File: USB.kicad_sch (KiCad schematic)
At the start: 31 parts, among them J5 USB_C_Receptacle, J6 USB_C_Receptacle, SW1 SW_DIP_x04, U10 TPS2552, U11 TPD4EUSB30, U12 TPD4EUSB30, U13 TPD4EUSB30, U14 TPD4EUSB30, U15 TS3USB221, U16 HD3SS3220, U17 TS3USB221

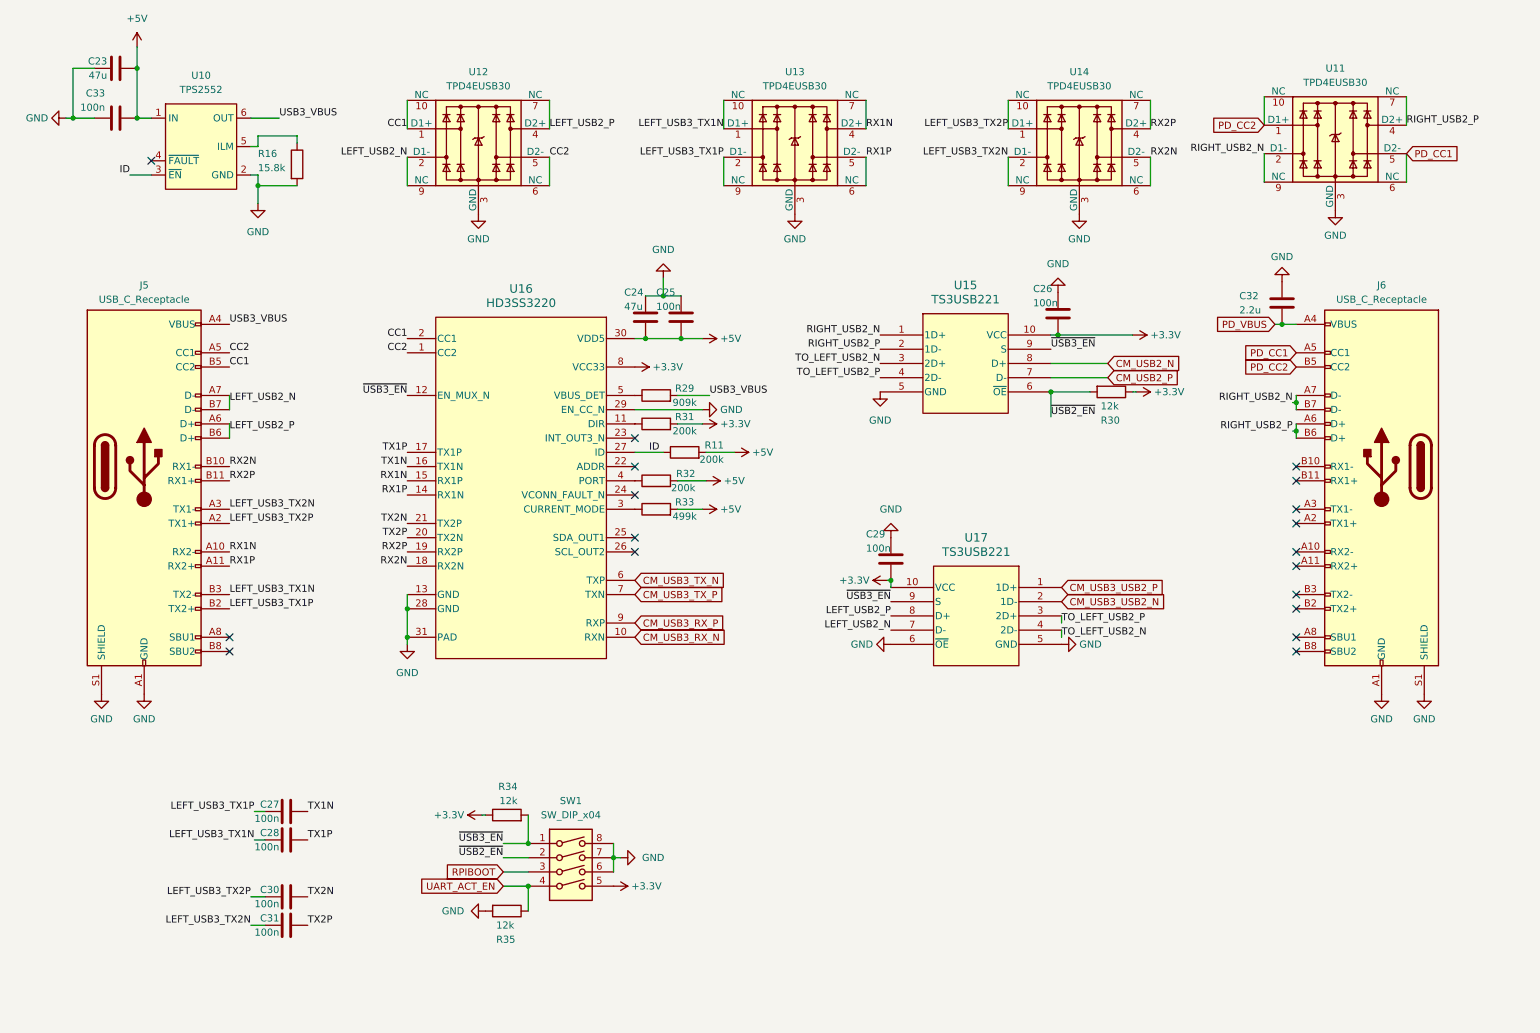
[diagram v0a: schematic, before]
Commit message: PiCard v3.0
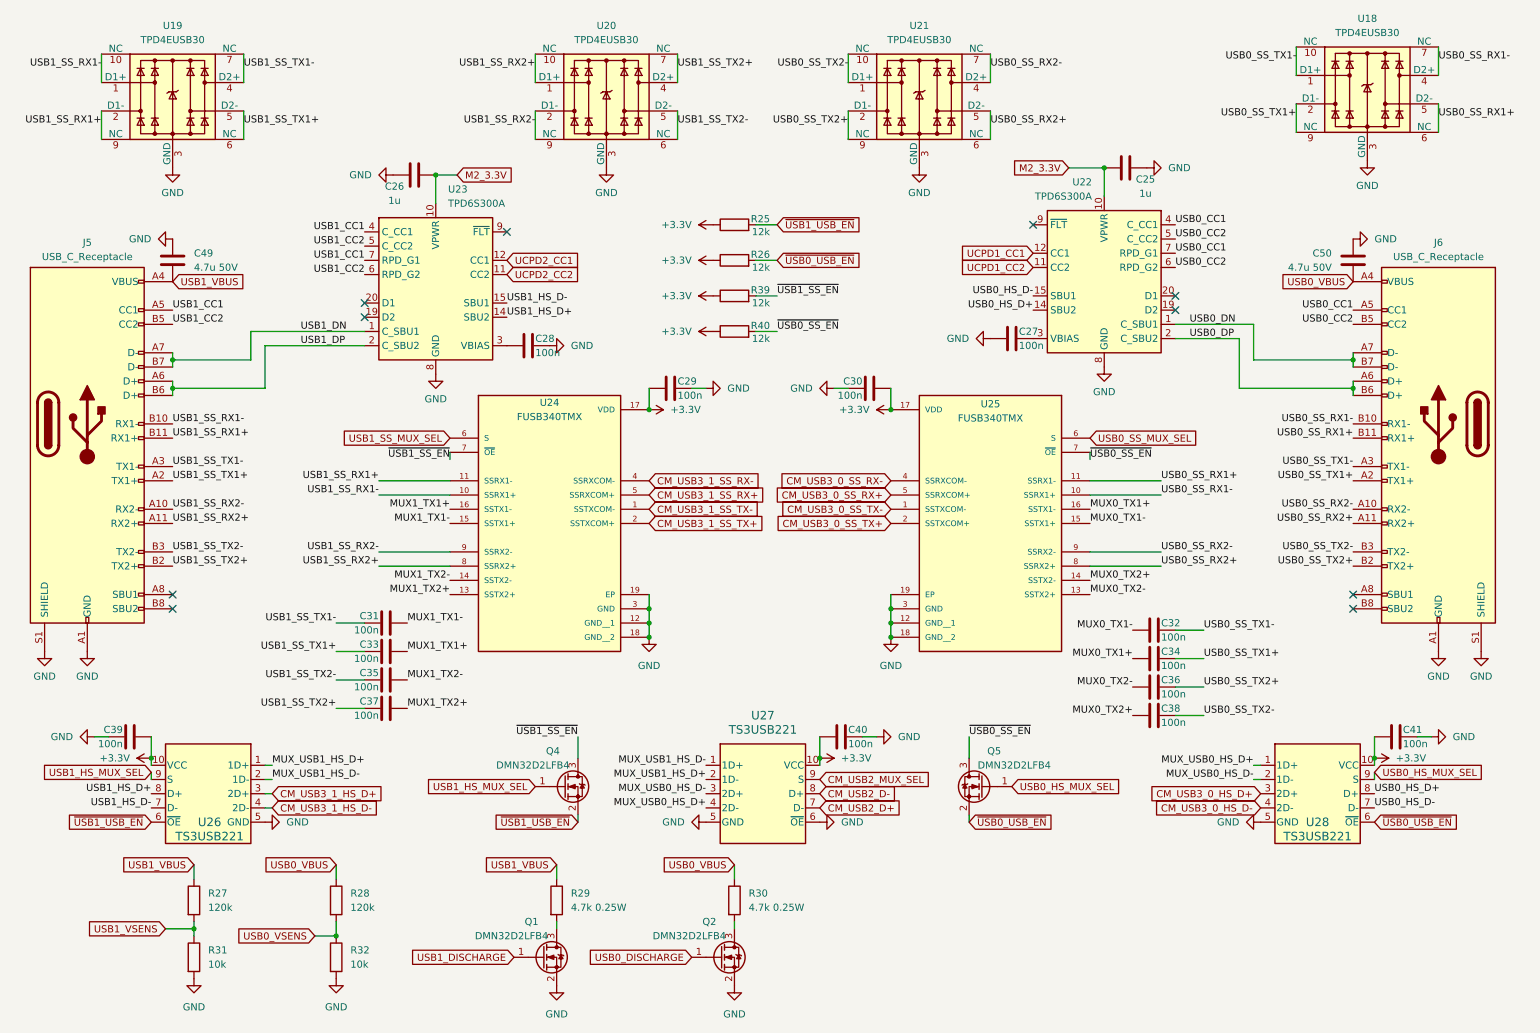
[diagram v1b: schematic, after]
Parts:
- removed C23, C24: 47u, Capacitor_SMD:C_0805_2012Metric, symbol Device:C
- removed R11: 200k, Resistor_SMD:R_0402_1005Metric, symbol Device:R
- removed R16: 15.8k, Resistor_SMD:R_0402_1005Metric, symbol Device:R
- removed R33: 499k, Resistor_SMD:R_0402_1005Metric, symbol Device:R
- removed R34, R35: 12k, Resistor_SMD:R_0402_1005Metric, symbol Device:R
- removed SW1: SW_DIP_x04, PiCard:SW-SMD_8P-P1.27_EU-04KS, symbol Switch:SW_DIP_x04
- removed U10: TPS2552, Package_TO_SOT_SMD:SOT-23-6, symbol PiCard:TPS2552
- removed U11, U12, U13: TPD4EUSB30, Package_SON:USON-10_2.5x1.0mm_P0.5mm, symbol Power_Protection:TPD4EUSB30
- removed U15, U17: TS3USB221, Package_DFN_QFN:Texas_UQFN-10_1.5x2mm_P0.5mm, symbol PiCard:TS3USB221
- removed U16: HD3SS3220, PiCard:RNH0030A, symbol PiCard:HD3SS3220
- added C34, C35, C36, C37, C38, C39, C40, C41: 100n, Capacitor_SMD:C_0402_1005Metric, symbol Device:C
- added C49, C50: 4.7u 50V, Capacitor_SMD:C_0805_2012Metric, symbol Device:C
- added Q1, Q2, Q4, Q5: DMN32D2LFB4, Package_DFN_QFN:Diodes_DFN1006-3, symbol Device:Q_NMOS_GSD
- added R25, R26, R39, R40: 12k, Resistor_SMD:R_0402_1005Metric, symbol Device:R
- added R27, R28: 120k, Resistor_SMD:R_0402_1005Metric, symbol Device:R
- added U18, U20, U21: TPD4EUSB30, Package_SON:USON-10_2.5x1.0mm_P0.5mm, symbol Power_Protection:TPD4EUSB30
- added U22, U23: TPD6S300A, Package_DFN_QFN:WQFN-20-1EP_3x3mm_P0.4mm_EP1.7x1.7mm_ThermalVias, symbol Power_Protection:TPD6S300A
- added U24, U25: FUSB340TMX, PiCard:QFN-18-1EP_2x2.8mm_P0.4mm_EP1.05x1.85mm, symbol PiCard:FUSB340TMX
- added U26, U27, U28: TS3USB221, PiCard:RSE10, symbol PiCard:TS3USB221
- C25, C26: value 100n -> 1u; footprint Capacitor_SMD:C_0402_1005Metric -> Capacitor_SMD:C_0603_1608Metric; LCSC C307331 -> C15849; MPN CL05B104KB54PNC -> CL10A105KB8NNNC
- C32: value 2.2u -> 100n; footprint Capacitor_SMD:C_1206_3216Metric -> Capacitor_SMD:C_0402_1005Metric; LCSC C50254 -> C307331; MPN CL31B225KBHNNNE -> CL05B104KB54PNC
- R29: value 909k -> 4.7k 0.25W; footprint Resistor_SMD:R_0402_1005Metric -> Resistor_SMD:R_1206_3216Metric; LCSC C2085054 -> C17936; MPN ERJ2RKF9093X -> 1206W4F4701T5E; Manufacturer PANASONIC -> Uniroyal
- R30: value 12k -> 4.7k 0.25W; footprint Resistor_SMD:R_0402_1005Metric -> Resistor_SMD:R_1206_3216Metric; LCSC C25752 -> C17936; MPN 0402WGF1202TCE -> 1206W4F4701T5E
- R31, R32: value 200k -> 10k; LCSC C25764 -> C25744; MPN 0402WGF2003TCE -> 0402WGF1002TCE
- renumbered U14 to U19
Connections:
- net TX1N is gone; now on net GND: C27.2
- net TX2N is gone; now on net +3.3V: C30.2
- net +3.3V: now also C39.2, C40.2, C41.2, R25.1, R26.1, R39.1, R40.1, U24.17 (VDD), U25.17 (VDD), U26.10 (VCC), U27.10 (VCC), U28.10 (VCC); no longer C26.2, R30.1, R31.2
- net GND: now also C28.1, C30.1, R31.2, R32.2, C39.1, C40.1, C41.1, C49.1, C50.1, Q1.2 (S), Q2.2 (S), U18.3 (GND), U18.8 (GND), U20.3 (GND), U20.8 (GND), U21.3 (GND), U21.8 (GND), U22.13 (GND), U22.16 (GND), U22.17 (GND), U22.18 (GND), U22.21 (GND), U22.8 (GND), U23.13 (GND), U23.16 (GND), U23.17 (GND), U23.18 (GND), U23.21 (GND), U23.8 (GND), U24.12 (GND__1), U24.18 (GND__2), U24.19 (EP), U24.3 (GND), U25.12 (GND__1), U25.18 (GND__2), U25.19 (EP), U25.3 (GND), U26.5 (GND), U27.5 (GND), U27.6 (~{OE}), U28.5 (GND); no longer C32.1, C33.1
- net USB1_VSENS: now reaches R31.1
- net USB1_VSENS: now also R27.2
- net USB1_VBUS: now reaches R29.1
- net USB1_VBUS: now also J5.A4 (VBUS), J5.A9 (VBUS), J5.B4 (VBUS), J5.B9 (VBUS), C49.2, R27.1
- net USB0_VSENS: now reaches R32.1
- net USB0_VSENS: now also R28.2
- net USB0_SS_RX2-: now reaches J6.A10 (RX2-)
- net USB0_SS_RX2-: now also U21.4 (D2+), U21.7 (NC), U25.9 (SSRX2-)
- net USB0_SS_RX2+: now reaches J6.A11 (RX2+)
- net USB0_SS_RX2+: now also U21.5 (D2-), U21.6 (NC), U25.8 (SSRX2+)
- net USB0_SS_TX1+: now reaches J6.A2 (TX1+)
- net USB0_SS_TX1+: now also C34.1, U18.2 (D1-), U18.9 (NC)
- net USB0_SS_TX1-: now reaches J6.A3 (TX1-)
- net USB0_SS_TX1-: now also C32.1, U18.1 (D1+), U18.10 (NC)
- net USB0_SS_RX1-: now reaches J6.B10 (RX1-)
- net USB0_SS_RX1-: now also U18.4 (D2+), U18.7 (NC), U25.10 (SSRX1+)
- net USB0_SS_RX1+: now reaches J6.B11 (RX1+)
- net USB0_SS_RX1+: now also U18.5 (D2-), U18.6 (NC), U25.11 (SSRX1-)
- net USB0_SS_TX2+: now reaches J6.B2 (TX2+)
- net USB0_SS_TX2+: now also C36.1, U21.2 (D1-), U21.9 (NC)
- net USB0_SS_TX2-: now reaches J6.B3 (TX2-)
- net USB0_SS_TX2-: now also C38.1, U21.1 (D1+), U21.10 (NC)
- removed net +5V: C25.2, C33.2, R32.2
- net CC1 renamed USB1_CC2
- net USB1_CC2: now also U23.5 (C_CC2), U23.6 (RPD_G2)
- net CC2 renamed USB1_CC1
- net USB1_CC1: now also U23.4 (C_CC1), U23.7 (RPD_G1)
- net LEFT_USB2_N renamed USB1_DN
- net USB1_DN: now also U23.1 (C_SBU1)
- net LEFT_USB2_P renamed USB1_DP
- net USB1_DP: now also U23.2 (C_SBU2)
- net LEFT_USB3_TX1N renamed USB1_SS_TX2-
- net USB1_SS_TX2-: now also C35.1, U20.5 (D2-), U20.6 (NC); no longer C28.1
- net LEFT_USB3_TX1P: no longer names the net of C27.1
- net LEFT_USB3_TX1P: now also U22.3 (VBIAS); no longer J5.B2 (TX2+)
- net LEFT_USB3_TX2N renamed USB1_SS_RX1+
- net USB1_SS_RX1+: now also J5.B11 (RX1+), U24.11 (SSRX1-); no longer C31.1, J5.A3 (TX1-)
- net LEFT_USB3_TX2P renamed USB1_SS_RX1-
- net USB1_SS_RX1-: now also J5.B10 (RX1-), U24.10 (SSRX1+); no longer C30.1, J5.A2 (TX1+)
- net PD_CC1 renamed USB0_CC1
- net USB0_CC1: now also U22.4 (C_CC1), U22.7 (RPD_G1)
- net PD_CC2 renamed USB0_CC2
- net USB0_CC2: now also U22.5 (C_CC2), U22.6 (RPD_G2)
- net PD_VBUS renamed USB0_VBUS
- net USB0_VBUS: now also R30.1, C50.2, R28.1; no longer C32.2
- net RIGHT_USB2_N renamed USB0_DN
- net USB0_DN: now also U22.1 (C_SBU1)
- net RIGHT_USB2_P renamed USB0_DP
- net USB0_DP: now also U22.2 (C_SBU2)
- net RX1N renamed USB1_SS_RX2-
- net USB1_SS_RX2-: now also U20.2 (D1-), U20.9 (NC), U24.9 (SSRX2-)
- net RX1P renamed USB1_SS_RX2+
- net USB1_SS_RX2+: now also U20.1 (D1+), U20.10 (NC), U24.8 (SSRX2+)
- net RX2N renamed USB1_SS_TX1+
- net USB1_SS_TX1+: now also C33.1, J5.A2 (TX1+); no longer J5.B10 (RX1-)
- net RX2P renamed USB1_SS_TX1-
- net USB1_SS_TX1-: now also C31.1, J5.A3 (TX1-); no longer J5.B11 (RX1+)
- net TX1P: no longer names the net of C28.2
- net TX1P: now also U23.3 (VBIAS)
- net TX2P renamed MUX1_TX1-
- net MUX1_TX1-: now also U24.15 (SSTX1+)
- removed net USB3_VBUS: J5.A4 (VBUS), J5.A9 (VBUS), J5.B4 (VBUS), J5.B9 (VBUS), R29.2
- net ~{USB2_EN}: no longer names the net of R30.2
- net ~{USB2_EN}: now also Q2.3 (D)
- new net: Q1.3 (D), R29.2
- new net CM_USB2_D+: U27.7 (D-)
- new net CM_USB2_D-: U27.8 (D+)
- new net CM_USB2_MUX_SEL: U27.9 (S)
- new net CM_USB3_0_HS_D+: U28.3 (2D+)
- new net CM_USB3_0_HS_D-: U28.4 (2D-)
- new net CM_USB3_0_SS_RX+: U25.5 (SSRXCOM+)
- new net CM_USB3_0_SS_RX-: U25.4 (SSRXCOM-)
- new net CM_USB3_0_SS_TX+: U25.2 (SSTXCOM+)
- new net CM_USB3_0_SS_TX-: U25.1 (SSTXCOM-)
- new net CM_USB3_1_HS_D+: U26.3 (2D+)
- new net CM_USB3_1_HS_D-: U26.4 (2D-)
- new net CM_USB3_1_SS_RX+: U24.5 (SSRXCOM+)
- new net CM_USB3_1_SS_RX-: U24.4 (SSRXCOM-)
- new net CM_USB3_1_SS_TX+: U24.2 (SSTXCOM+)
- new net CM_USB3_1_SS_TX-: U24.1 (SSTXCOM-)
- new net M2_3.3V: C25.2, C26.2, U22.10 (VPWR), U23.10 (VPWR)
- new net MUX0_TX1+: C34.2, U25.16 (SSTX1-)
- new net MUX0_TX1-: C32.2, U25.15 (SSTX1+)
- new net MUX0_TX2+: C38.2, U25.14 (SSTX2-)
- new net MUX0_TX2-: C36.2, U25.13 (SSTX2+)
- new net MUX1_TX1+: C33.2, U24.16 (SSTX1-)
- new net MUX1_TX2+: C37.2, U24.13 (SSTX2+)
- new net MUX1_TX2-: C35.2, U24.14 (SSTX2-)
- new net MUX_USB0_HS_D+: U27.4 (2D-), U28.1 (1D+)
- new net MUX_USB0_HS_D-: U27.3 (2D+), U28.2 (1D-)
- new net MUX_USB1_HS_D+: U26.1 (1D+), U27.2 (1D-)
- new net MUX_USB1_HS_D-: U26.2 (1D-), U27.1 (1D+)
- new net UCPD1_CC1: U22.12 (CC1)
- new net UCPD1_CC2: U22.11 (CC2)
- new net UCPD2_CC1: U23.12 (CC1)
- new net UCPD2_CC2: U23.11 (CC2)
- new net USB0_DISCHARGE: Q2.1 (G)
- new net USB0_HS_D+: U22.14 (SBU2), U28.8 (D+)
- new net USB0_HS_D-: U22.15 (SBU1), U28.7 (D-)
- new net USB0_HS_MUX_SEL: Q5.1 (G), U28.9 (S)
- new net USB0_SS_MUX_SEL: U25.6 (S)
- new net USB1_DISCHARGE: Q1.1 (G)
- new net USB1_HS_D+: U23.14 (SBU2), U26.8 (D+)
- new net USB1_HS_D-: U23.15 (SBU1), U26.7 (D-)
- new net USB1_HS_MUX_SEL: Q4.1 (G), U26.9 (S)
- new net USB1_SS_MUX_SEL: U24.6 (S)
- new net USB1_SS_TX2+: C37.1, J5.B2 (TX2+), U20.4 (D2+), U20.7 (NC)
- new net ~{USB0_SS_EN}: Q5.3 (D), R40.2, U25.7 (~{OE})
- new net ~{USB0_USB_EN}: Q5.2 (S), R26.2, U28.6 (~{OE})
- new net ~{USB1_SS_EN}: Q4.3 (D), R39.2, U24.7 (~{OE})
- new net ~{USB1_USB_EN}: Q4.2 (S), R25.2, U26.6 (~{OE})
- no-connect marks 18 -> 10
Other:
- title: (none) -> PiCard
- moved on the sheet: J5, J6, U19
